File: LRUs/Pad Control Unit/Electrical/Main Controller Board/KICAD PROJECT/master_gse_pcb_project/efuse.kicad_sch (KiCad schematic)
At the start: 19 parts, among them J4 B2B-XH-A, U3 TPS259830ONRGER

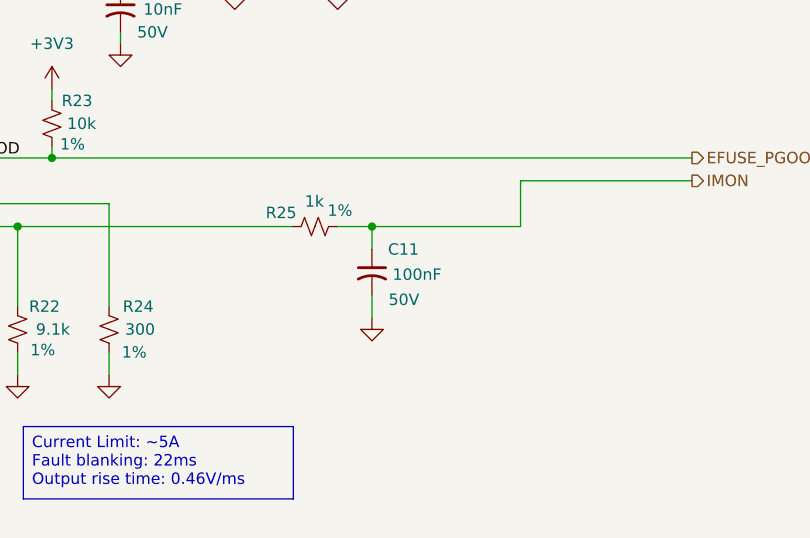
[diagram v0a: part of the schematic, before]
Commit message: Committ latest changes
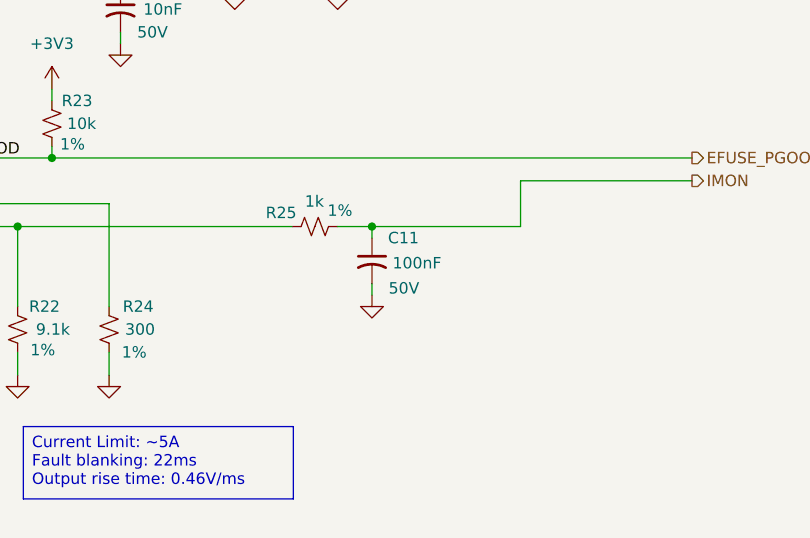
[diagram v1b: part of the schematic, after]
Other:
- moved on the sheet: C11
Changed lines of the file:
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@@
 	)
 	(junction
-		(at 220.98 97.79)
-		(diameter 0)
-		(color 0 0 0 0)
-	)
-	(junction
 		(at 185.42 90.17)
 		(diameter 0)
@@
 		(color 0 0 0 0)
 	)
+	(junction
+		(at 220.98 97.79)
+		(diameter 0)
+		(color 0 0 0 0)
+	)
 	(wire
 		(pts
@@
 	(wire
 		(pts
-			(xy 220.98 105.41) (xy 220.98 107.95)
+			(xy 220.98 104.14) (xy 220.98 105.41)
 		)
 		(stroke
@@
 	(wire
 		(pts
-			(xy 220.98 100.33) (xy 220.98 97.79)
+			(xy 220.98 99.06) (xy 220.98 97.79)
 		)
 		(stroke
@@
 	(symbol
 		(lib_id "Device:C_Small_US")
-		(at 220.98 102.87 0)
+		(at 220.98 101.6 0)
 		(unit 1)
 		(body_style 1)
@@
 		(dnp no)
 		(property "Reference" "C11"
-			(at 222.758 100.33 0)
+			(at 222.758 99.06 0)
 			(show_name no)
 			(do_not_autoplace no)
@@
 		)
 		(property "Value" "100nF"
-			(at 223.266 103.124 0)
+			(at 223.266 101.854 0)
 			(show_name no)
 			(do_not_autoplace no)
@@
 		)
 		(property "Footprint" "Capacitor_SMD:C_0402_1005Metric"
-			(at 220.98 102.87 0)
+			(at 220.98 101.6 0)
 			(hide yes)
 			(show_name no)
@@
 		)
 		(property "Datasheet" ""
-			(at 220.98 102.87 0)
+			(at 220.98 101.6 0)
 			(hide yes)
 			(show_name no)
@@
 		)
 		(property "Description" "100nF 50V X7R ±10% 0402 Capacitor"
-			(at 220.98 102.87 0)
+			(at 220.98 101.6 0)
 			(hide yes)
 			(show_name no)
@@
 		)
 		(property "Vmax" "50V"
-			(at 224.536 105.918 0)
+			(at 224.536 104.648 0)
 			(show_name no)
 			(do_not_autoplace no)
@@
 		)
 		(property "JLCPCB Part #" "C307331"
-			(at 220.98 102.87 0)
+			(at 220.98 101.6 0)
 			(hide yes)
 			(show_name no)
@@
 	(symbol
 		(lib_id "power:GND")
-		(at 220.98 107.95 0)
+		(at 220.98 105.41 0)
 		(unit 1)
 		(body_style 1)
@@
 		(fields_autoplaced yes)
 		(property "Reference" "#PWR035"
-			(at 220.98 114.3 0)
+			(at 220.98 111.76 0)
 			(hide yes)
 			(show_name no)
@@
 		)
 		(property "Value" "GND"
-			(at 220.98 113.03 0)
+			(at 220.98 110.49 0)
 			(hide yes)
 			(show_name no)
@@
 		)
 		(property "Footprint" ""
-			(at 220.98 107.95 0)
+			(at 220.98 105.41 0)
 			(hide yes)
 			(show_name no)
@@
 		)
 		(property "Datasheet" ""
-			(at 220.98 107.95 0)
+			(at 220.98 105.41 0)
 			(hide yes)
 			(show_name no)
@@
 		)
 		(property "Description" "Power symbol creates a global label with name \"GND\" , ground"
-			(at 220.98 107.95 0)
+			(at 220.98 105.41 0)
 			(hide yes)
 			(show_name no)
